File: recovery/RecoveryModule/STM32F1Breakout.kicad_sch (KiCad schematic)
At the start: 7 parts, among them U1 STM32F103C8Tx, U2 CP2102N-Axx-xQFN28

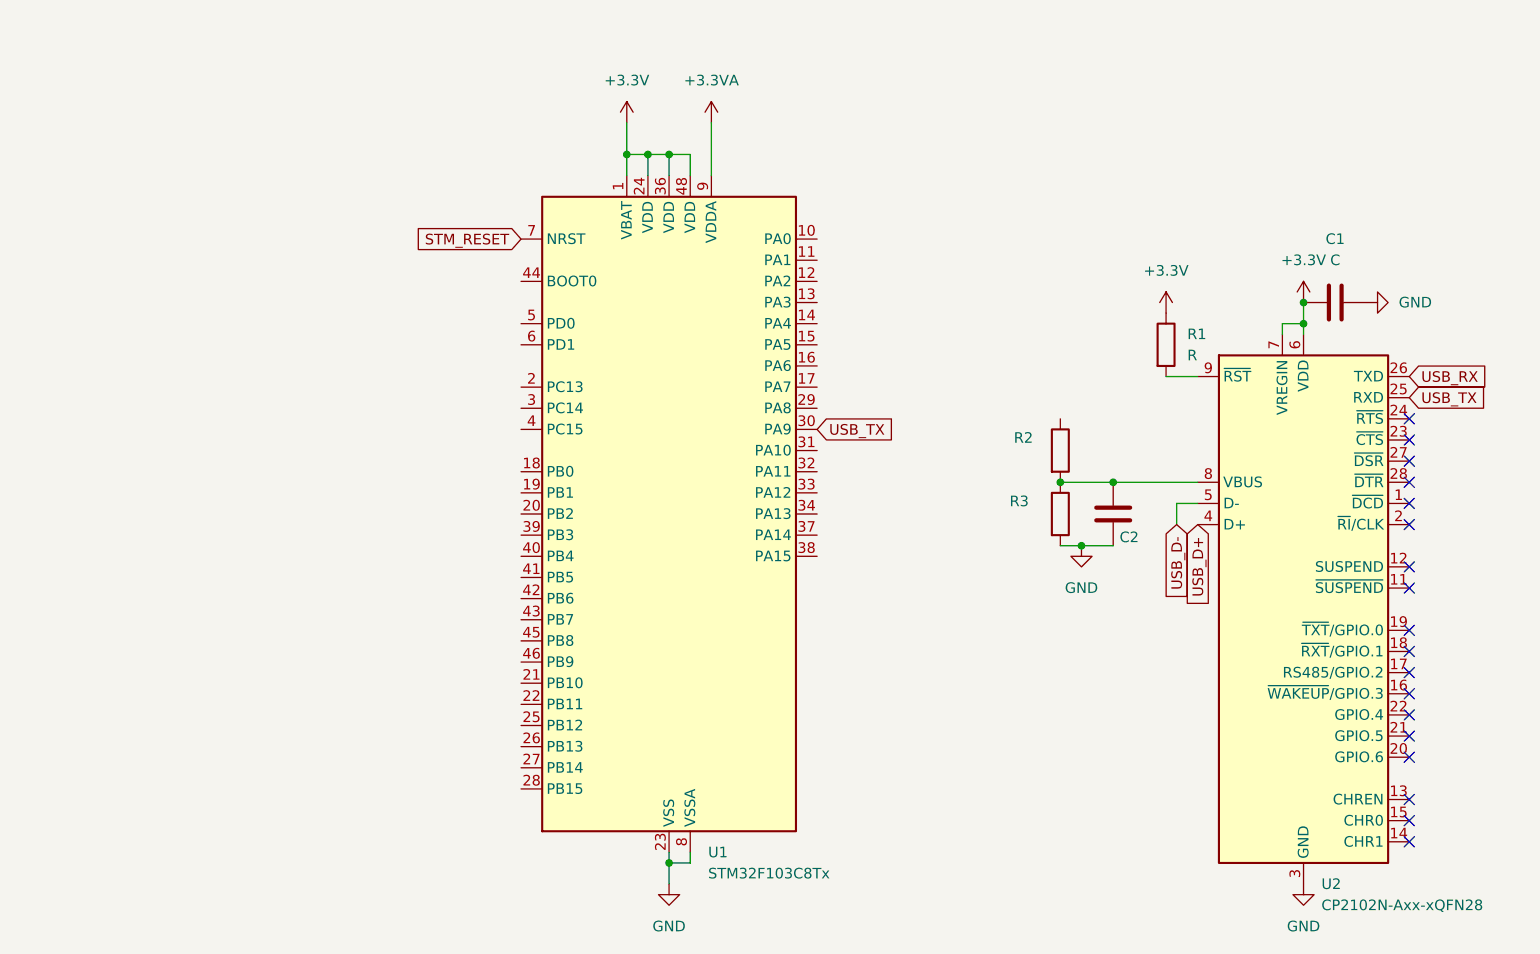
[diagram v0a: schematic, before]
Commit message: charge control schematics
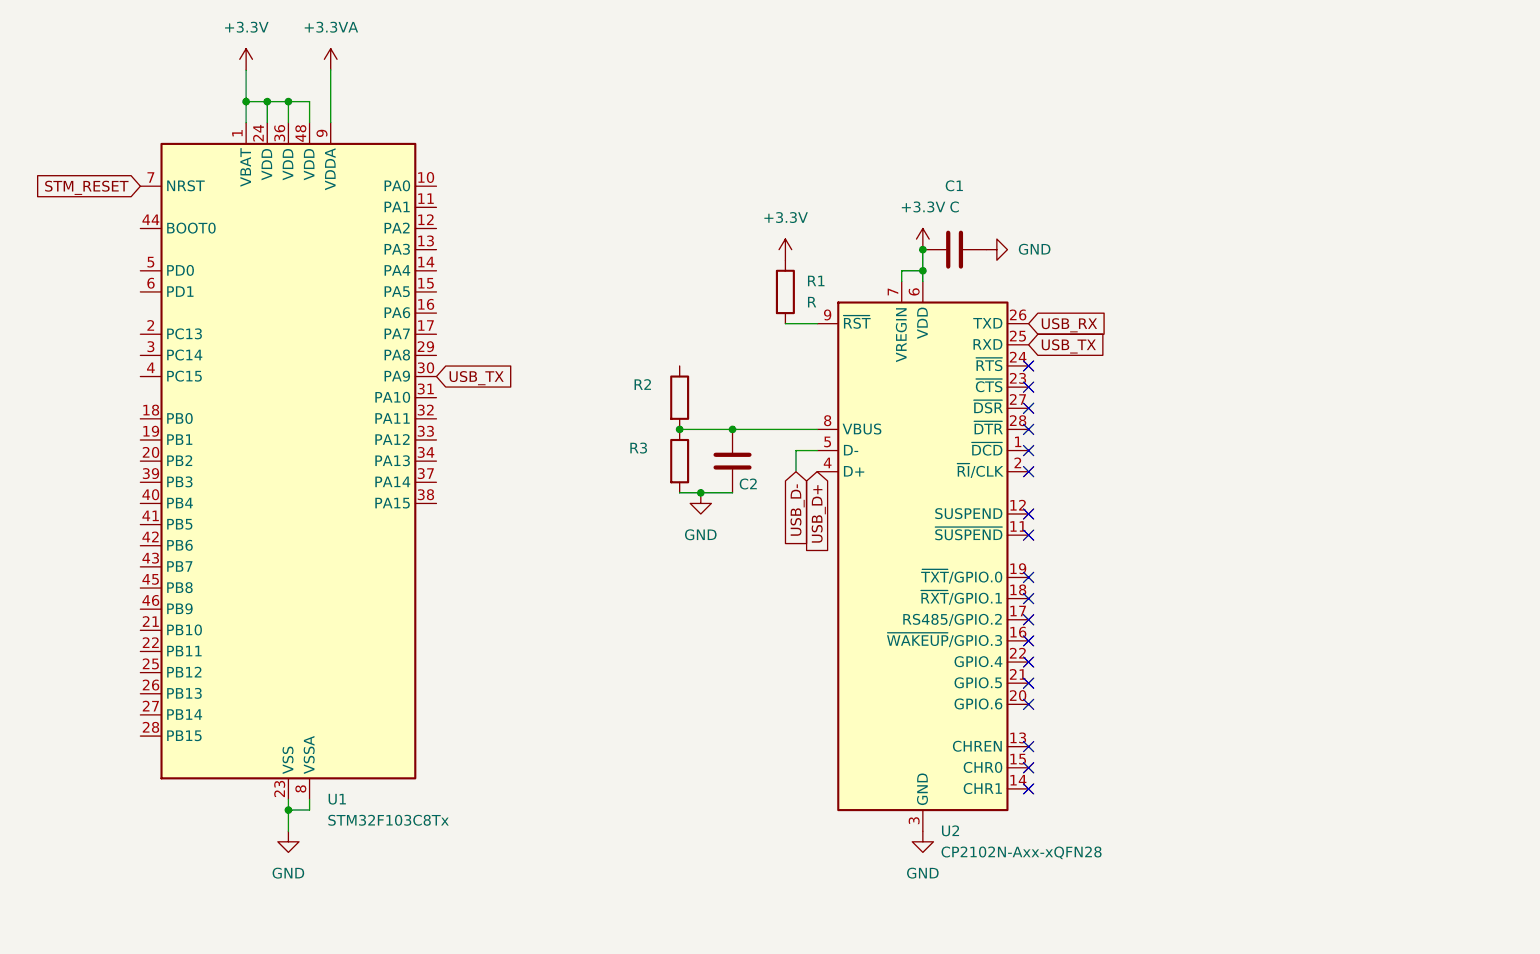
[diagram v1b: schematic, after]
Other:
- moved on the sheet: C1, C2, R1, R2, R3, U1, U2
